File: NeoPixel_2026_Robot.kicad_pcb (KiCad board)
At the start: 2 copper layers, 31 parts, among them J1 Pixcel1, J10 XT30, J2 Pixcel2, J3 Pixcel3, J4 Pixcel4, J5 INPUT, J6 EM-IN1, J7 EM-IN2, J8 EM-IN3, J9 EM-IN4, U1 TLP291, U2 TLP291, U3 TLP291, U4 TLP291

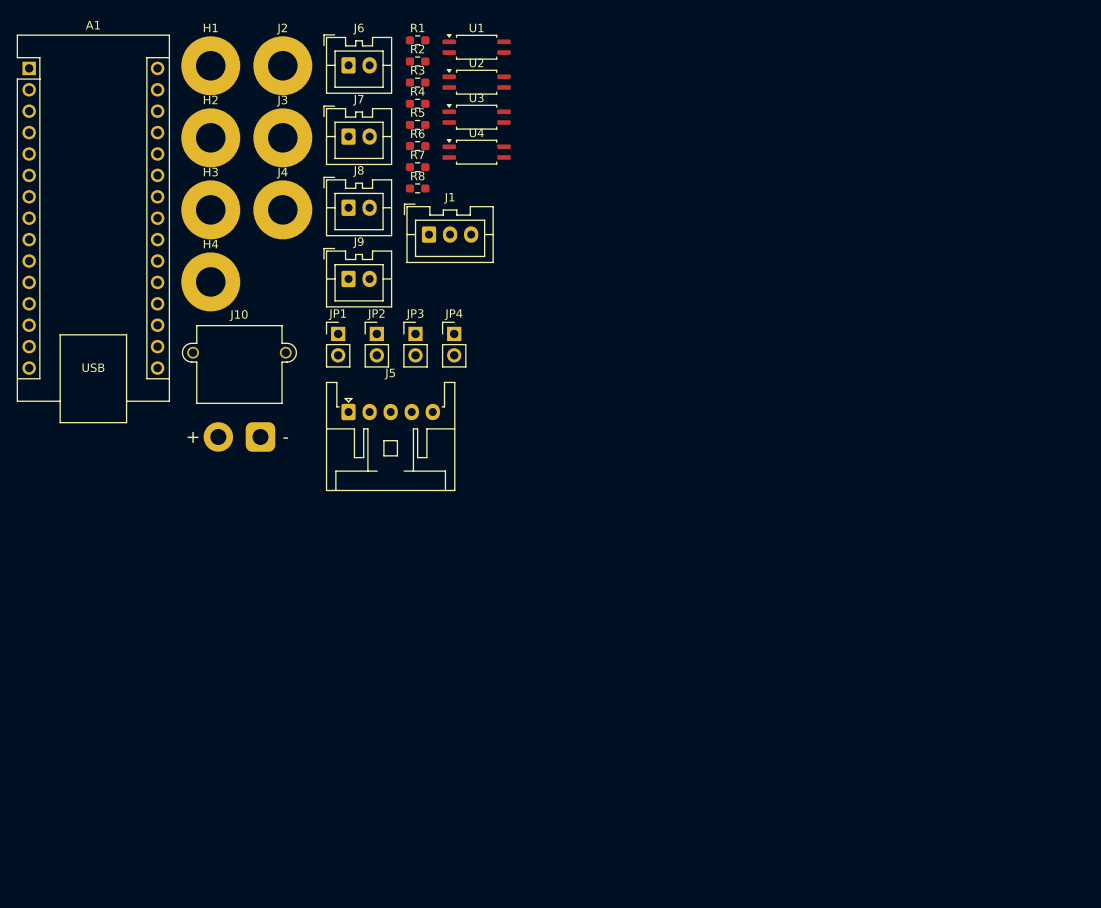
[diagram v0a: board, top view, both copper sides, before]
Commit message: おためし
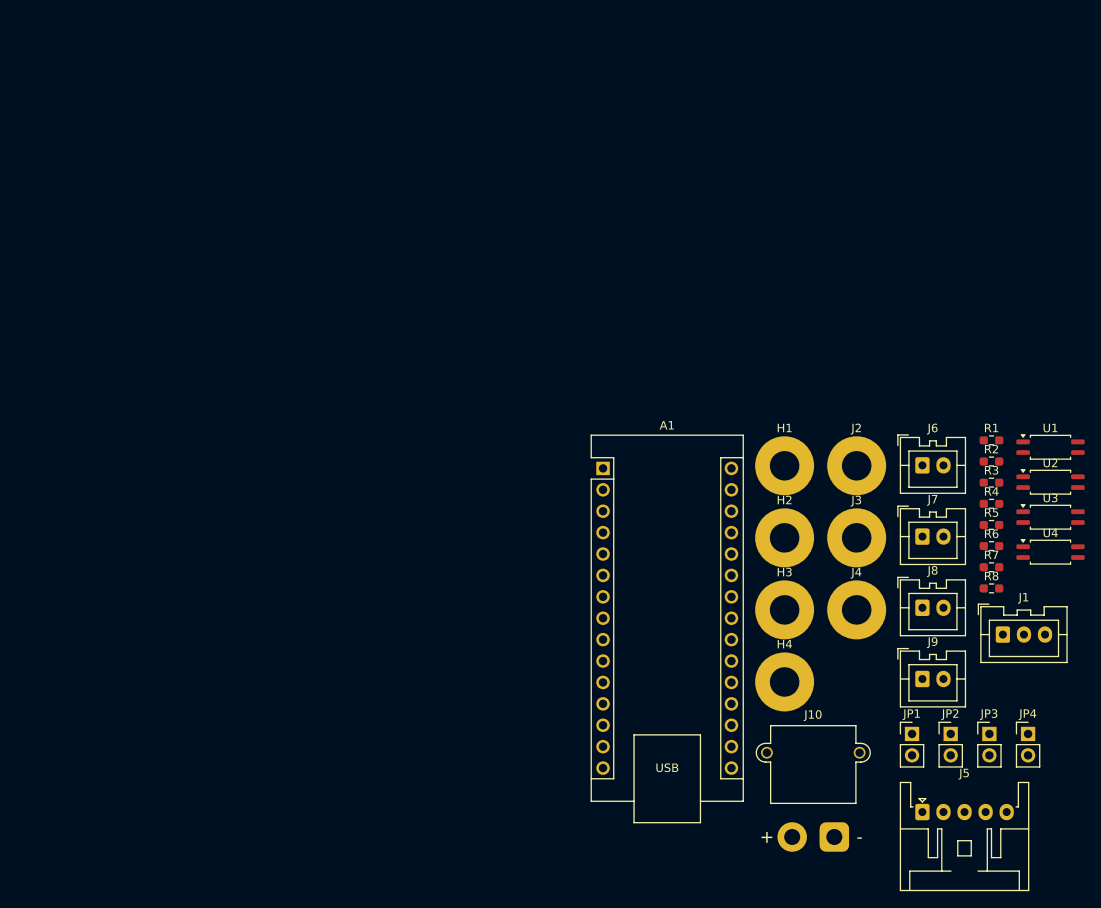
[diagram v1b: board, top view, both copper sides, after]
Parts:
- moved H3 83.0 mm to (91.4, 68.0)
- moved JP4 83.0 mm to (120.3, 82.7)
- moved A1 83.0 mm to (69.8, 51.2)
- moved H1 83.0 mm to (91.4, 50.9)
- moved H2 83.0 mm to (91.4, 59.5)
- moved H4 83.0 mm to (91.4, 76.6)
- moved J1 83.0 mm to (117.3, 70.9)
- moved J2 83.0 mm to (100.0, 50.9)
- moved J3 83.0 mm to (100.0, 59.5)
- moved J4 83.0 mm to (100.0, 68.0)
- moved J5 83.0 mm to (107.8, 92.0)
- moved J6 83.0 mm to (107.8, 50.9)
- moved J7 83.0 mm to (107.8, 59.3)
- moved J8 83.0 mm to (107.8, 67.8)
- moved J9 83.0 mm to (107.8, 76.2)
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
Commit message: windowsのほうで作ってたところまで手動復元
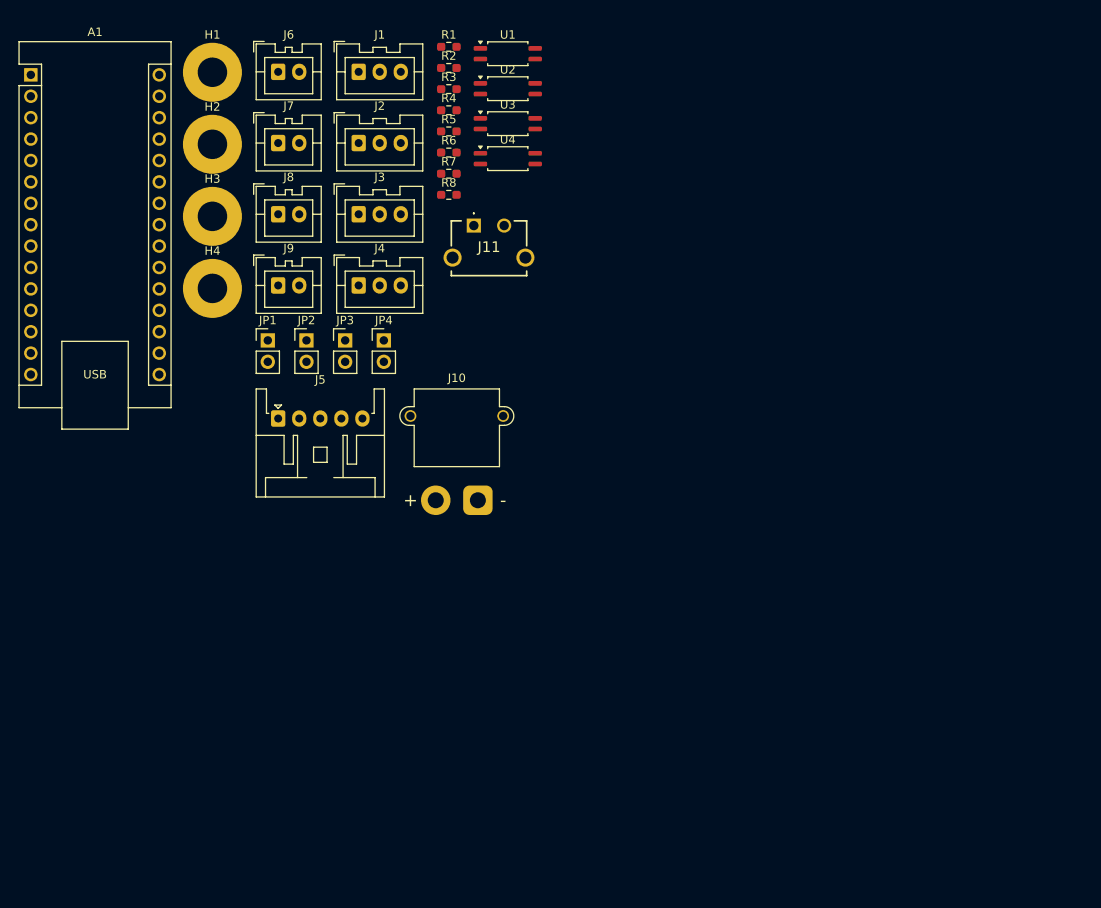
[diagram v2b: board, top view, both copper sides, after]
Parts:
- added J11: Type-C, NeoPixcel_2026_Robot_Lib:PowerOnlyUSB_C, F.Cu at (54.5, 22.4)
- J2, J3, J4: footprint MountingHole:MountingHole_3.5mm_Pad -> Connector_JST:JST_XA_B03B-XASK-1_1x03_P2.50mm_Vertical
- moved J1 101.5 mm to (40.9, 4.16)
- moved J5 89.6 mm to (31.3, 45.3)
- moved J6 89.6 mm to (31.3, 4.16)
- moved J7 89.6 mm to (31.3, 12.6)
- moved J8 89.6 mm to (31.3, 21.1)
- moved J9 89.6 mm to (31.3, 29.5)
- moved JP2 89.6 mm to (34.7, 36.0)
- moved JP3 89.6 mm to (39.2, 36.0)
- moved JP4 89.6 mm to (43.8, 36.0)
- moved JP1 89.6 mm to (30.1, 36.0)
- moved H1 82.4 mm to (23.5, 4.21)
- moved H2 82.4 mm to (23.5, 12.8)
- moved H3 82.4 mm to (23.5, 21.3)
- moved H4 82.4 mm to (23.5, 29.9)
- moved A1 82.4 mm to (1.95, 4.52)
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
